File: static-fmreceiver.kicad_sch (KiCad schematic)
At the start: 21 parts, among them CN1 PJ-3200, J1 Conn_01x02 (SPKR_R), J2 Conn_01x02 (SPKR_L), SW1 SW_Push, SW2 SW_Push, U1 RDA5807MRRD-102V2.0, U2 XIAO-RP2040-DIP, U3 TDA2822NBD

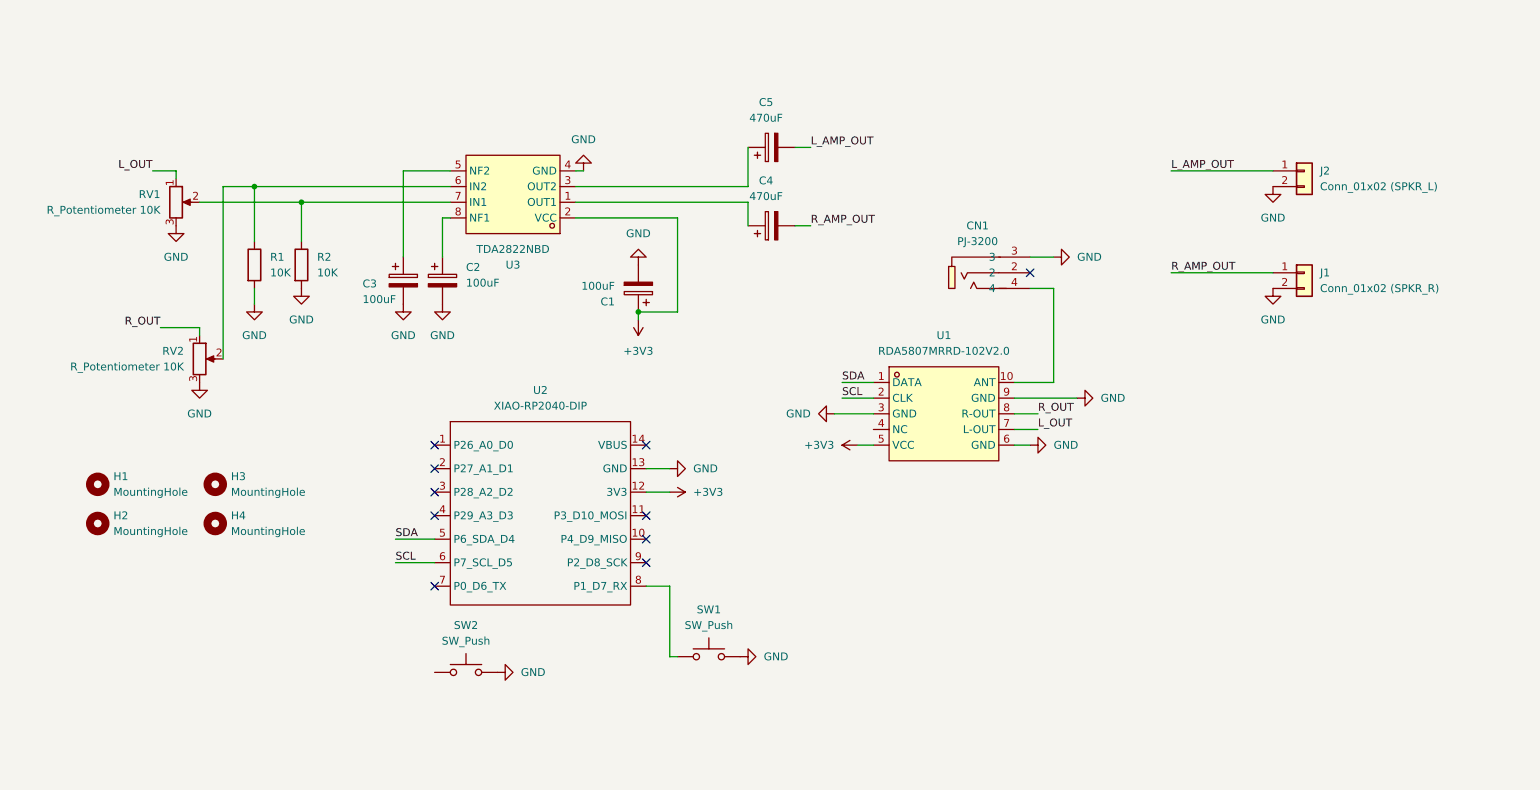
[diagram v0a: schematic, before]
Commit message: done with pcb methink
lots of silkscreen and optimised routing. I think it looks kinda nice
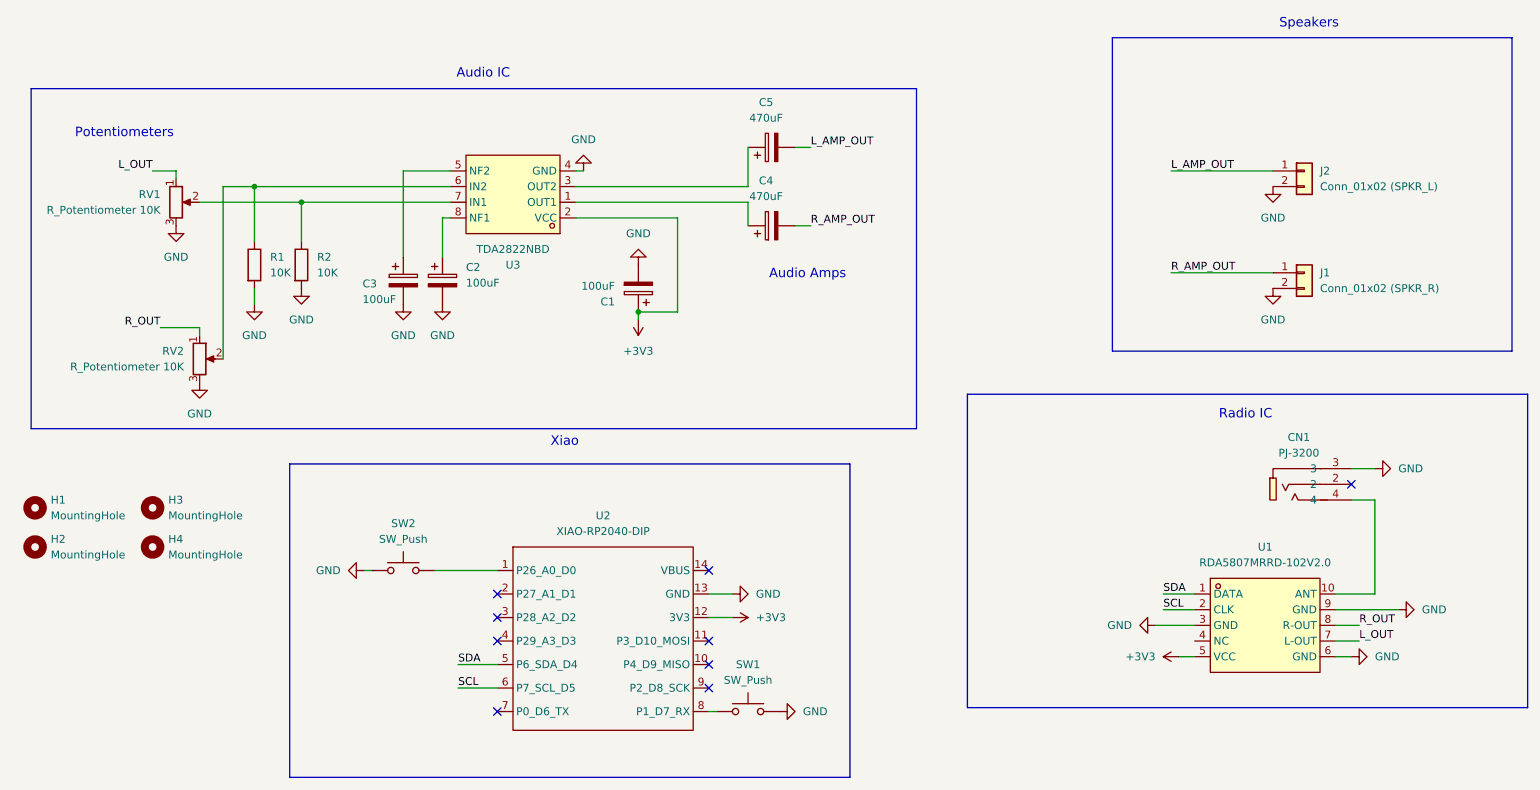
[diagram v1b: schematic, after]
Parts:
- CN1: footprint easyeda2kicad:AUDIO-TH_PJ-3200 -> Static:AUDIO-TH_PJ-3200
- SW2: footprint Button_Switch_Keyboard:SW_Cherry_MX_1.00u_PCB -> Connector_PinHeader_2.54mm:PinHeader_1x02_P2.54mm_Vertical
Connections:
- net GND: now also SW2.1; no longer SW2.2
- net at U2.1 (P26_A0_D0): now also SW2.2
- no-connect marks 10 -> 9
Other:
- note added: "Audio Amps"
- note added: "Audio IC"
- note added: "Potentiometers"
- note added: "Radio IC"
- note added: "Speakers"
- note added: "Xiao"
- moved on the sheet: CN1, H1, H2, H3, H4, SW1, SW2, U1, U2
